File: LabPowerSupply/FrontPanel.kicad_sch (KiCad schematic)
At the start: 27 parts, among them SW11 Decimal, SW12 0, SW13 Backspace, SW14 Current 2, SW15 Cancel, SW21 1, SW22 2, SW23 3, SW24 Voltage 2, SW25 Confirm, SW31 4, SW32 5, SW33 6, SW34 Current 1, SW35 Channel 2, SW41 7, SW42 8, SW43 9, SW44 Voltage 1, SW45 Channel 1

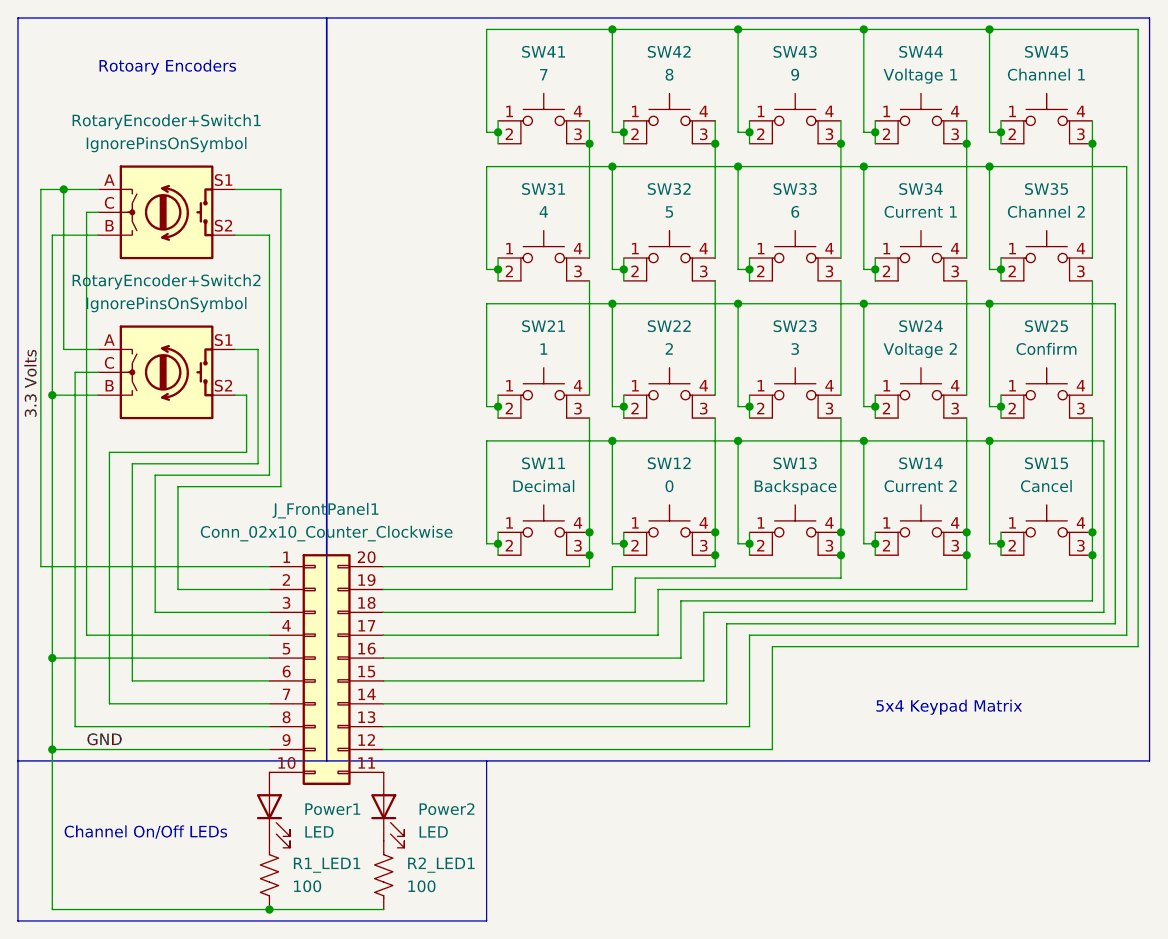
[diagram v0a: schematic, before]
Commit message: Start tallying
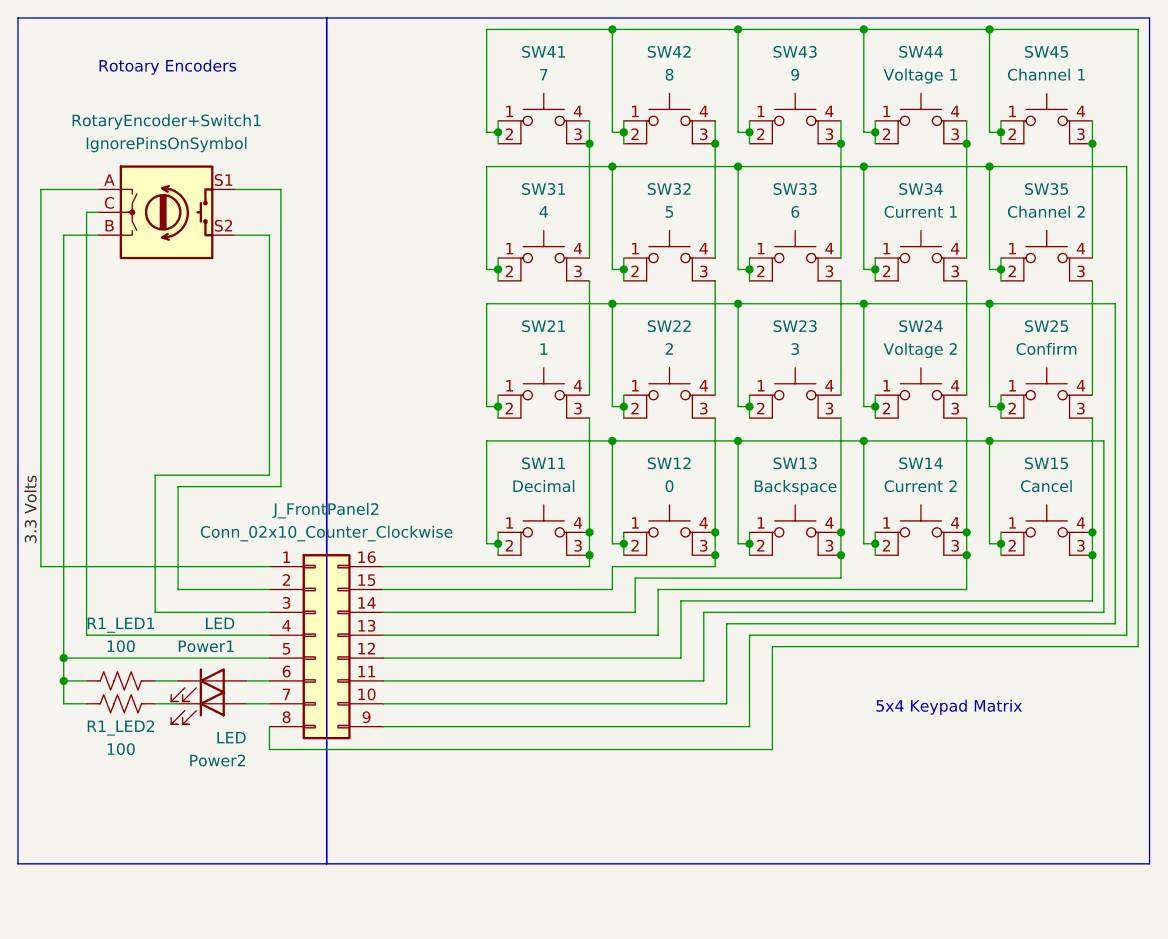
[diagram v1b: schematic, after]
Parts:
- removed J_FrontPanel1: Conn_02x10_Counter_Clockwise, Connector_IDC:IDC-Header_2x10_P2.54mm_Vertical, symbol Connector_Generic:Conn_02x10_Counter_Clockwise
- removed R2_LED1: 100, Resistor_SMD:R_0603_1608Metric, symbol Device:R_US
- removed RotaryEncoder+Switch2: IgnorePinsOnSymbol, Rotary_Encoder:RotaryEncoder_Alps_EC11E-Switch_Vertical_H20mm, symbol Device:RotaryEncoder_Switch
- added J_FrontPanel2: Conn_02x10_Counter_Clockwise, Connector_IDC:IDC-Header_2x10_P2.54mm_Vertical, symbol Connector_Generic:Conn_02x08_Counter_Clockwise
- added R1_LED2: 100, Resistor_SMD:R_0603_1608Metric, symbol Device:R_US
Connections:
- net 3.3 Volts: now also J_FrontPanel2.1 (Pin_1)
- net at SW31.1, SW31.2, SW32.1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: now also J_FrontPanel2.9 (Pin_9)
- net at SW11.1, SW11.2, SW12.1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: now also J_FrontPanel2.11 (Pin_11)
- net at SW12.3 (K), SW12.4 (A), SW22.3 (K): now also J_FrontPanel2.15 (Pin_15)
- net at Power1.2 (A): now also J_FrontPanel2.6 (Pin_6)
- net at Power2.2 (A): now also J_FrontPanel2.7 (Pin_7)
- net at SW41.1, SW41.2, SW42.1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: now also J_FrontPanel2.8 (Pin_8)
- net at SW21.1, SW21.2, SW22.1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: now also J_FrontPanel2.10 (Pin_10)
- net at SW15.3 (K), SW15.4 (A), SW25.3 (K): now also J_FrontPanel2.12 (Pin_12)
- net at SW14.3 (K), SW14.4 (A), SW24.3 (K): now also J_FrontPanel2.13 (Pin_13)
- net at SW13.3 (K), SW13.4 (A), SW23.3 (K): now also J_FrontPanel2.14 (Pin_14)
- net at RotaryEncoder+Switch1.S1: now also J_FrontPanel2.2 (Pin_2)
- net at SW11.3 (K), SW11.4 (A), SW21.3 (K): now also J_FrontPanel2.16 (Pin_16)
- net at RotaryEncoder+Switch1.S2: now also J_FrontPanel2.3 (Pin_3)
- net at RotaryEncoder+Switch1.C: now also J_FrontPanel2.4 (Pin_4)
- net at Power2.1 (K): now also R1_LED2.1
- net GND: no longer names the net of R1_LED1.2, RotaryEncoder+Switch1.B
- net GND: now also J_FrontPanel2.5 (Pin_5), R1_LED2.2
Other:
- note removed: "Channel On/Off LEDs"
